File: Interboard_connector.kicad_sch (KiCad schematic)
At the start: 2 parts, among them J1 Chainbus In, J2 Chainbus Out

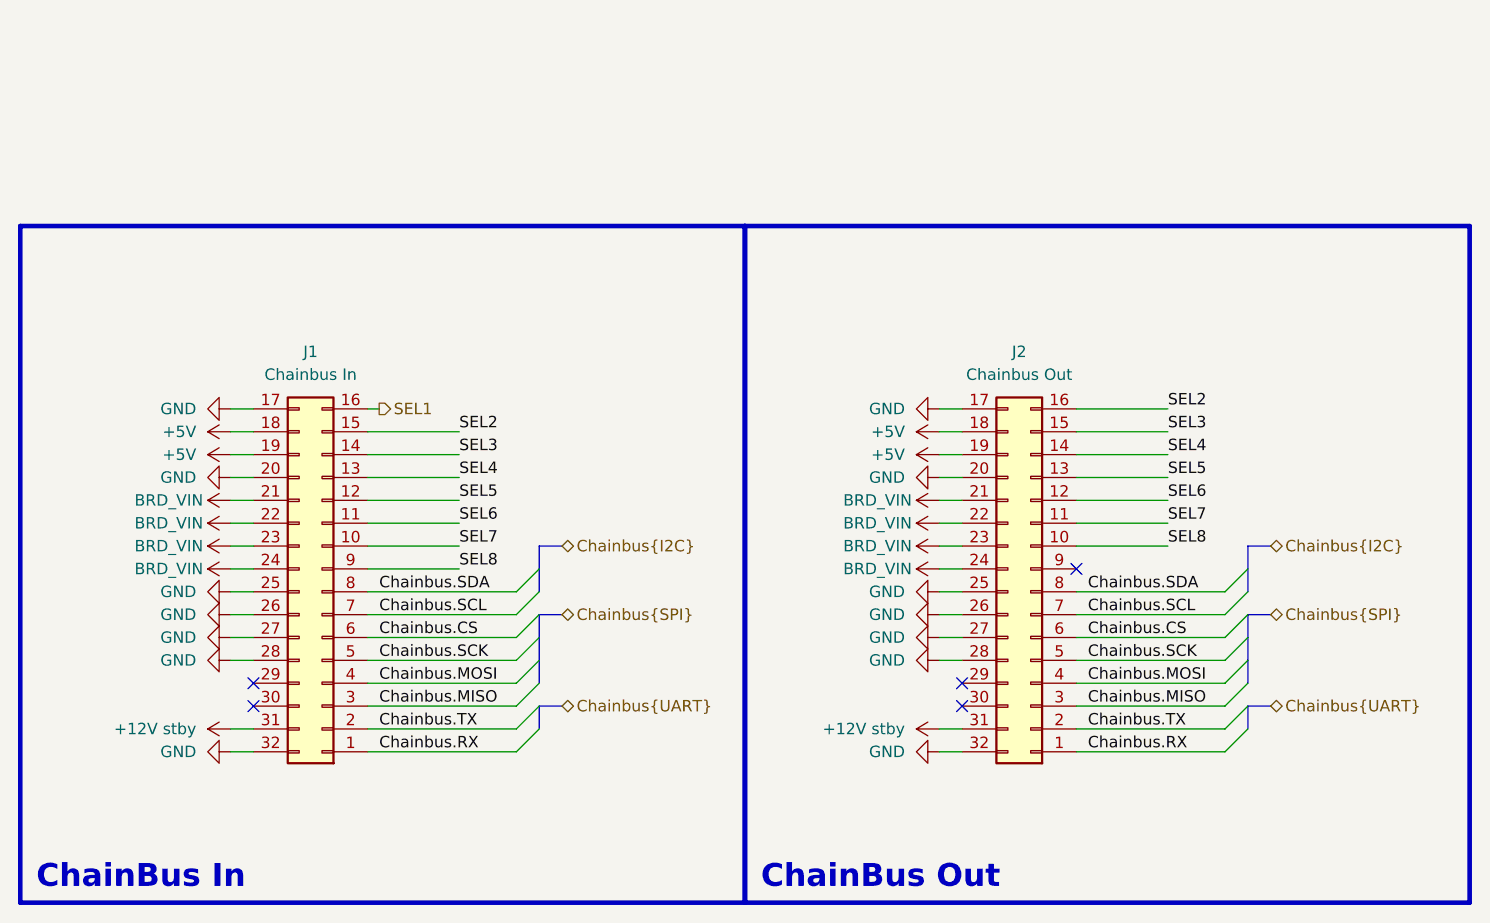
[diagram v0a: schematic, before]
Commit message: revision
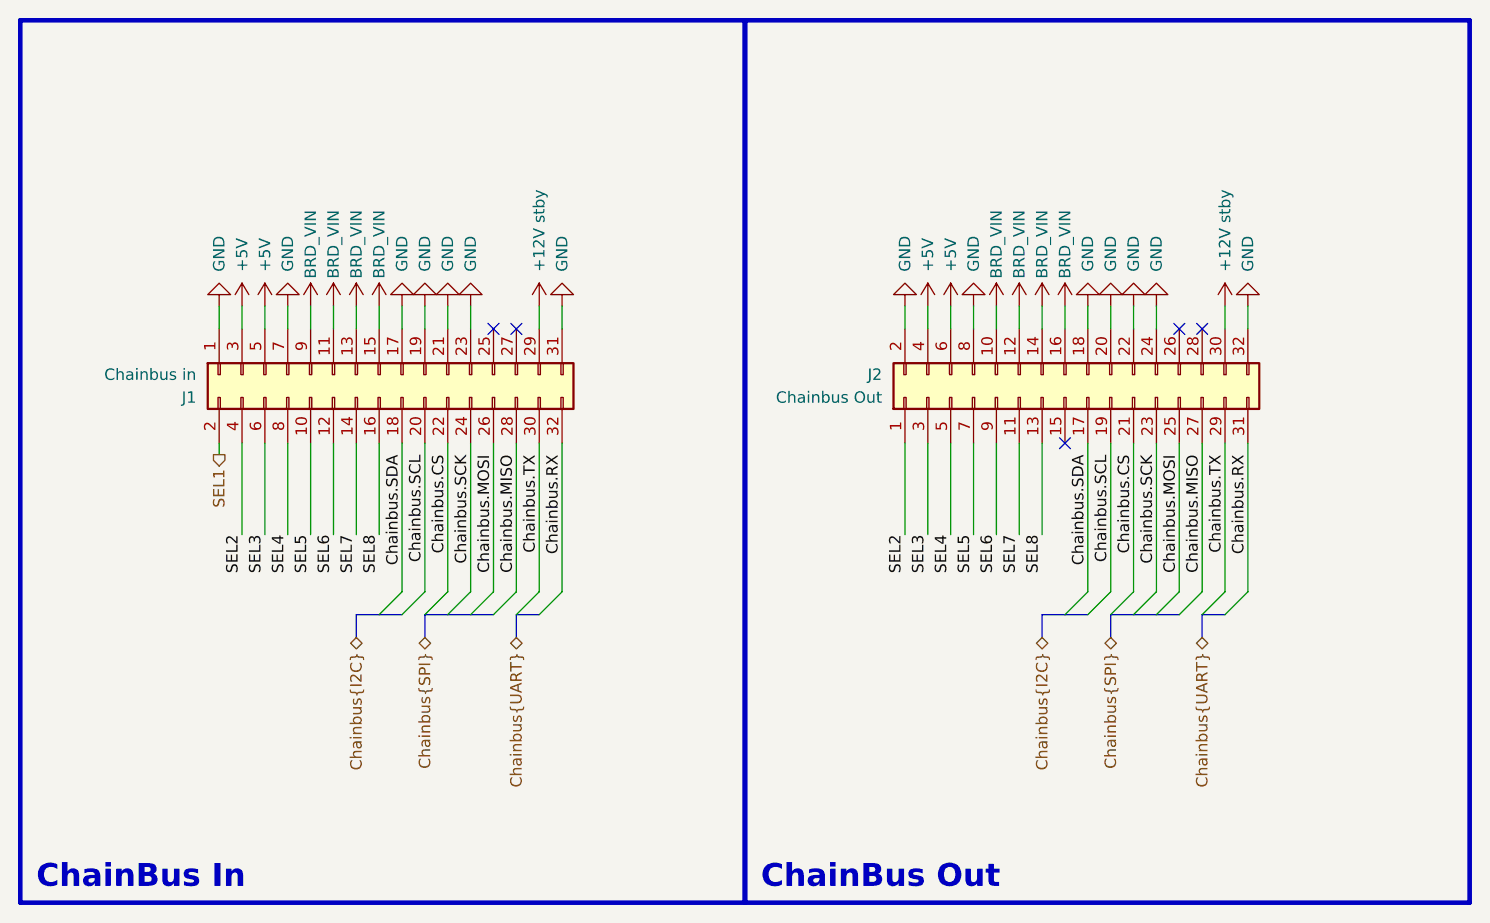
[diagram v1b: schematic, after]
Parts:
- removed J1: Chainbus In, Connector_PinSocket_2.54mm:PinSocket_2x16_P2.54mm_Vertical_SMD, symbol Connector_Generic:Conn_02x16_Counter_Clockwise
- removed J2: Chainbus Out, Connector_PinSocket_2.54mm:PinSocket_2x16_P2.54mm_Vertical_SMD, symbol Connector_Generic:Conn_02x16_Counter_Clockwise
- added J1: Chainbus in, Connector_PinSocket_2.54mm:PinSocket_2x16_P2.54mm_Vertical_SMD, symbol Connector_Generic:Conn_02x16_Odd_Even
- added J2: Chainbus Out, Connector_PinSocket_2.54mm:PinSocket_2x16_P2.54mm_Vertical_SMD, symbol Connector_Generic:Conn_02x16_Odd_Even
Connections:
- net +12V stby: now also J1.29 (Pin_29), J2.30 (Pin_30)
- net +5V: now also J1.3 (Pin_3), J1.5 (Pin_5), J2.4 (Pin_4), J2.6 (Pin_6)
- net BRD_VIN: now also J1.11 (Pin_11), J1.13 (Pin_13), J1.15 (Pin_15), J1.9 (Pin_9), J2.10 (Pin_10), J2.12 (Pin_12), J2.14 (Pin_14), J2.16 (Pin_16)
- net Chainbus.CS: now also J1.22 (Pin_22), J2.21 (Pin_21)
- net Chainbus.MISO: now also J1.28 (Pin_28), J2.27 (Pin_27)
- net Chainbus.MOSI: now also J1.26 (Pin_26), J2.25 (Pin_25)
- net Chainbus.RX: now also J1.32 (Pin_32), J2.31 (Pin_31)
- net Chainbus.SCK: now also J1.24 (Pin_24), J2.23 (Pin_23)
- net Chainbus.SCL: now also J1.20 (Pin_20), J2.19 (Pin_19)
- net Chainbus.SDA: now also J1.18 (Pin_18), J2.17 (Pin_17)
- net Chainbus.TX: now also J1.30 (Pin_30), J2.29 (Pin_29)
- net GND: now also J1.1 (Pin_1), J1.17 (Pin_17), J1.19 (Pin_19), J1.21 (Pin_21), J1.23 (Pin_23), J1.31 (Pin_31), J1.7 (Pin_7), J2.18 (Pin_18), J2.2 (Pin_2), J2.20 (Pin_20), J2.22 (Pin_22), J2.24 (Pin_24), J2.32 (Pin_32), J2.8 (Pin_8)
- net SEL1: now also J1.2 (Pin_2)
- net SEL2: now also J1.4 (Pin_4), J2.1 (Pin_1)
- net SEL3: now also J1.6 (Pin_6), J2.3 (Pin_3)
- net SEL4: now also J1.8 (Pin_8), J2.5 (Pin_5)
- net SEL5: now also J1.10 (Pin_10), J2.7 (Pin_7)
- net SEL6: now also J1.12 (Pin_12), J2.9 (Pin_9)
- net SEL7: now also J1.14 (Pin_14), J2.11 (Pin_11)
- net SEL8: now also J1.16 (Pin_16), J2.13 (Pin_13)
